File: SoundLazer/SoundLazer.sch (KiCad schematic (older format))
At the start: 133 parts, among them J1 Audio_in, J2 DSP_PROG, J3 PWR_SEL, J4 12V_IN, J5 SPK_OUT, Q1 ZXTP25040DZTA, Q2 MMDT2222V, Q3 MMDT2907V, Q4 FDS4935A, Q5 FDS6890A, Q6 2N7002, Q7 2N7002, Q8 2N7002, SW1 EG1381A, SW2 EG1381A, U1 24AA256-I/SN, U2 TL494, U3 HEF4049BT,653, U4 ADAU1701, U5 MC78M06CDTRKG, U6 AZ1117-3.3, U7 CAT811STBI-GT3, Y1 ABM8-12.288MHZ-B2-T

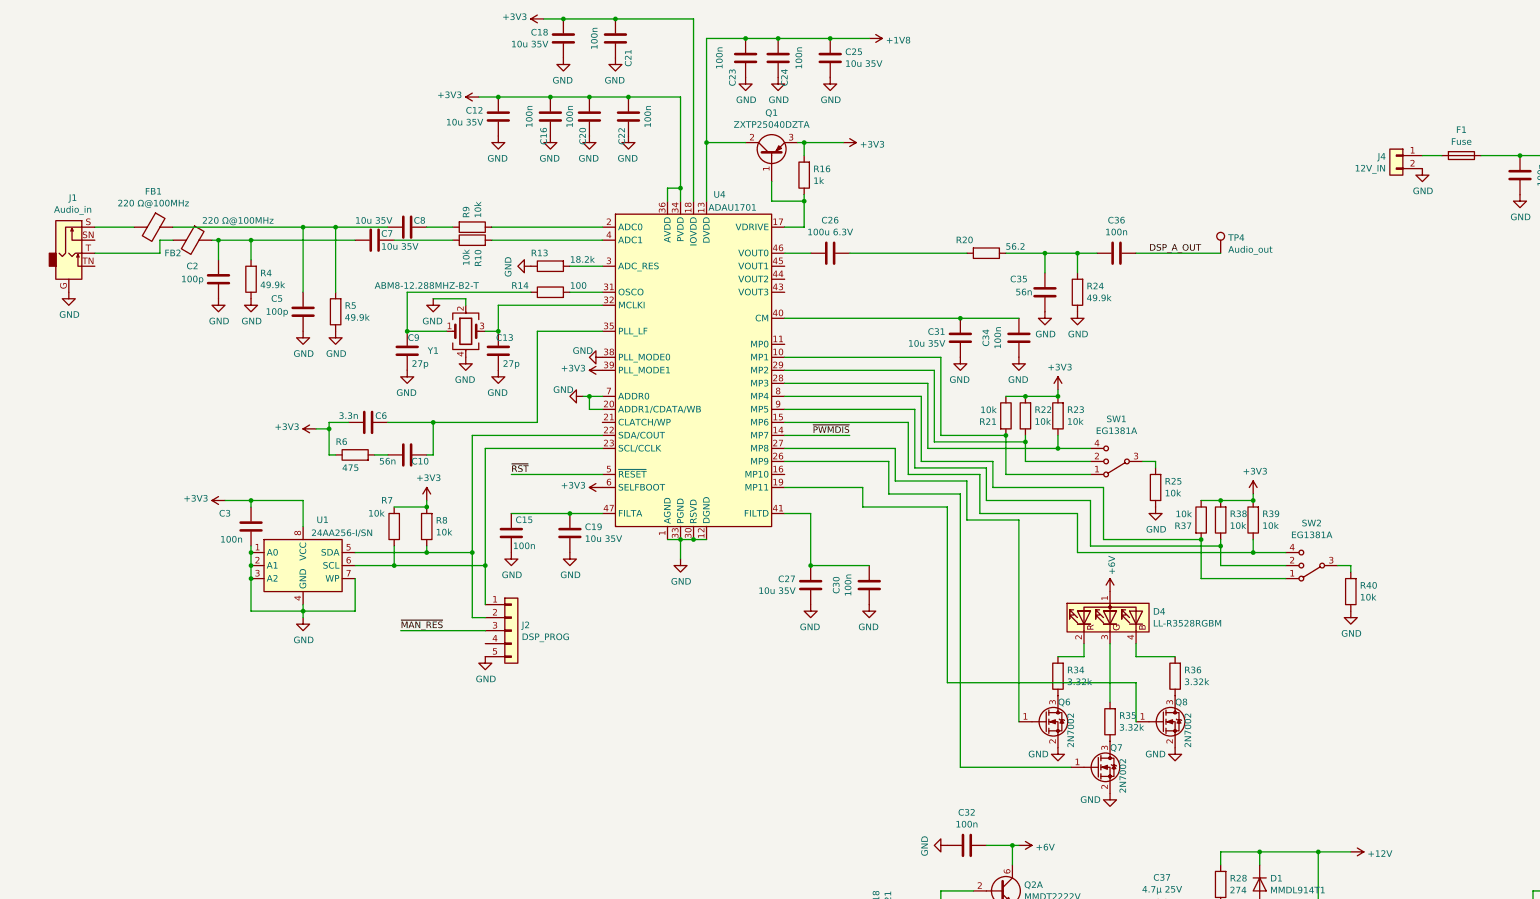
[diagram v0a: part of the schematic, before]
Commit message: pcb_finish
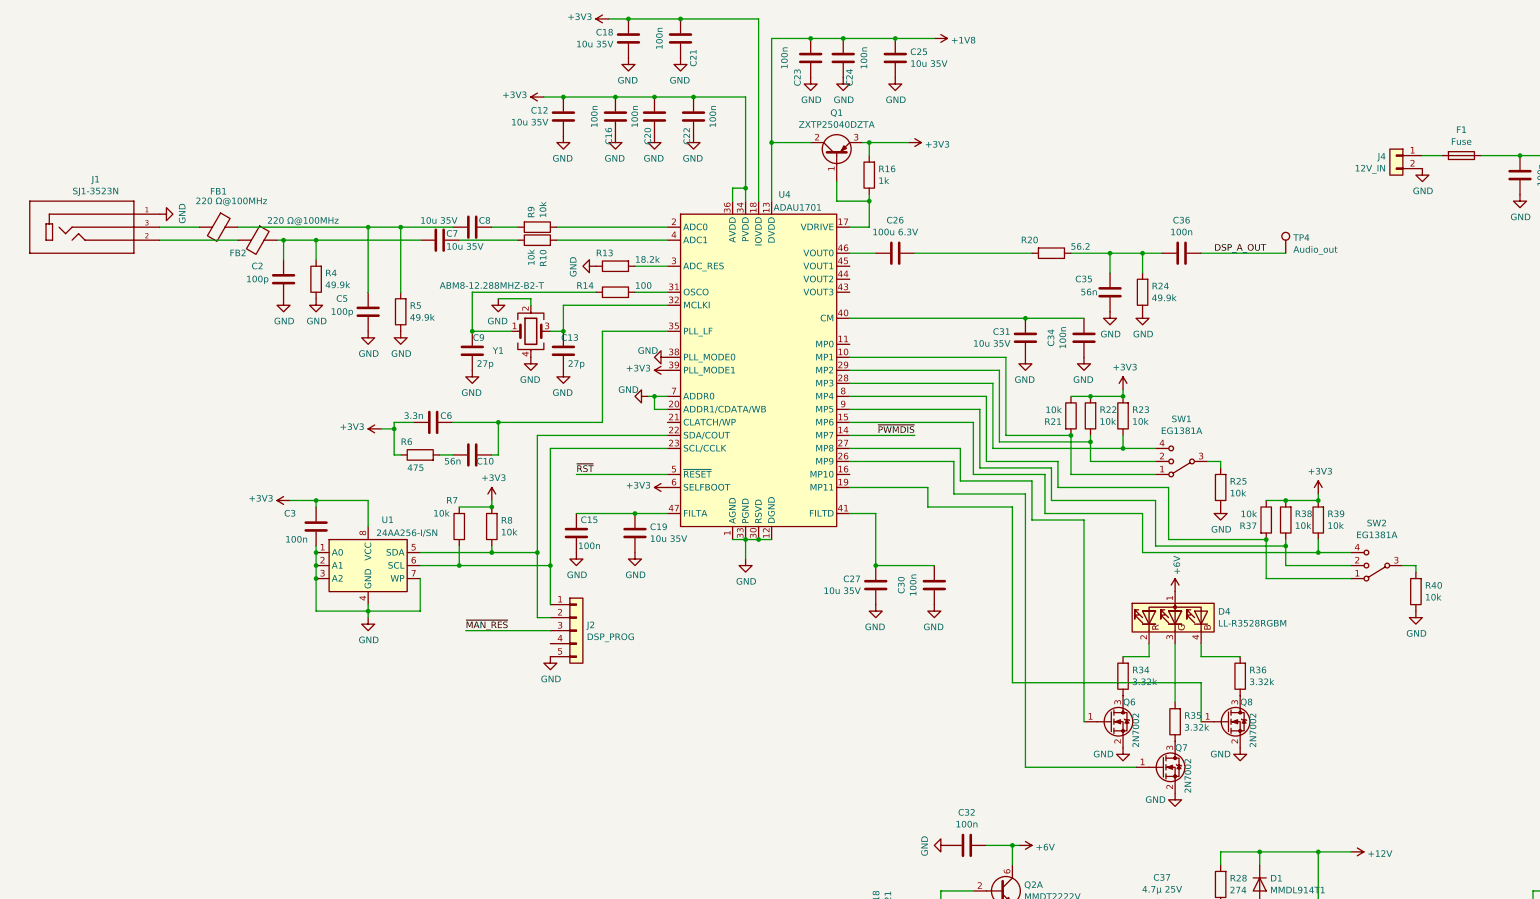
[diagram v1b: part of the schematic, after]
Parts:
- removed J1: Audio_in, Connector_Audio:Jack_3.5mm_Ledino_KB3SPRS_Horizontal, symbol Connector:AudioJack2_Ground_Switch
- added J1: SJ1-3523N, temp_pcb_lib:CUI_SJ1-3523N, symbol SJ1-3523N:SJ1-3523N
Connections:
- net GND: now also J1.1
- net at FB1.2: now also J1.3
- net at FB2.2: now also J1.2
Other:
- moved on the sheet: C10, C12, C13, C15, C16, C18, C19, C2, C20, C21, C22, C23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
